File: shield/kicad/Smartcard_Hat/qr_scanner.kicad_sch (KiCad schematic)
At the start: 7 parts, among them J10 SFV12R-2STE1HLF

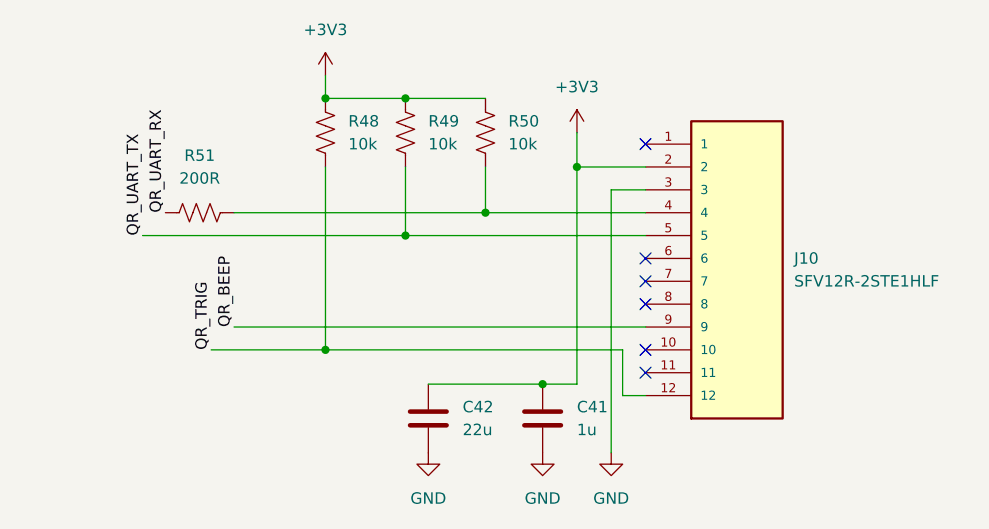
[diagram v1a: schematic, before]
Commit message: wip
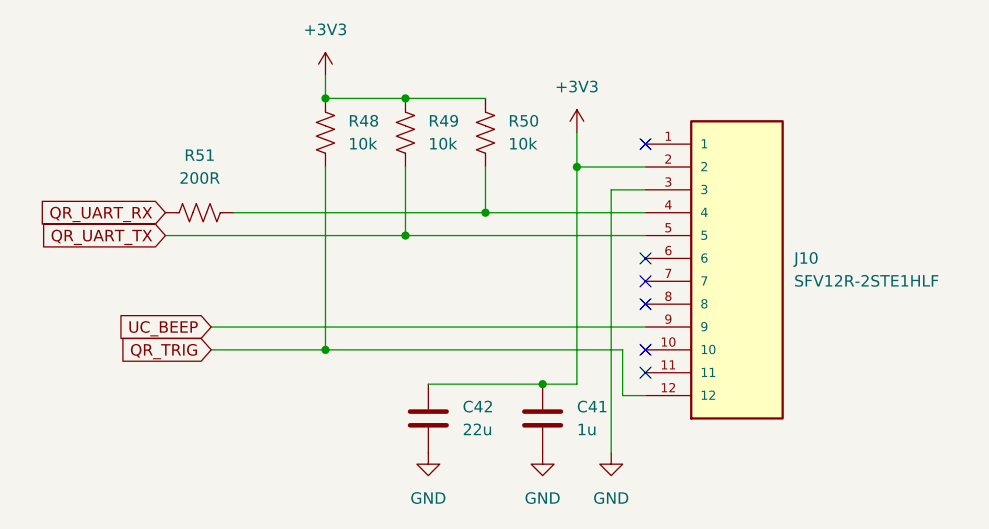
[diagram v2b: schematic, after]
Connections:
- net QR_BEEP renamed UC_BEEP
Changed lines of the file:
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@@
+	(wire
+		(pts
+			(xy 124.46 101.6) (xy 172.72 101.6)
+		)
+		(stroke
+			(width 0)
+			(type default)
+		)
+	)
 	(wire
 		(pts
@@
 	(wire
 		(pts
-			(xy 127 101.6) (xy 172.72 101.6)
-		)
-		(stroke
-			(width 0)
-			(type default)
-		)
-	)
-	(wire
-		(pts
 			(xy 127 88.9) (xy 154.94 88.9)
 		)
@@
 	(wire
 		(pts
-			(xy 116.84 91.44) (xy 146.05 91.44)
+			(xy 119.38 91.44) (xy 146.05 91.44)
 		)
 		(stroke
@@
 		)
 	)
-	(label "QR_UART_RX"
-		(at 119.38 88.9 90)
-		(fields_autoplaced yes)
-		(effects
-			(font
-				(size 1.27 1.27)
-			)
-			(justify left bottom)
-		)
-	)
-	(label "QR_TRIG"
-		(at 124.46 104.14 90)
-		(fields_autoplaced yes)
-		(effects
-			(font
-				(size 1.27 1.27)
-			)
-			(justify left bottom)
-		)
-	)
-	(label "QR_BEEP"
-		(at 127 101.6 90)
-		(fields_autoplaced yes)
-		(effects
-			(font
-				(size 1.27 1.27)
-			)
-			(justify left bottom)
-		)
-	)
-	(label "QR_UART_TX"
-		(at 116.84 91.44 90)
-		(fields_autoplaced yes)
-		(effects
-			(font
-				(size 1.27 1.27)
-			)
-			(justify left bottom)
-		)
-	)
+	(global_label "UC_BEEP"
+		(shape input)
+		(at 124.46 101.6 180)
+		(fields_autoplaced yes)
+		(effects
+			(font
+				(size 1.27 1.27)
+			)
+			(justify right)
+		)
+		(property "Intersheetrefs" "${INTERSHEET_REFS}"
+			(at 112.9736 101.6 0)
+			(effects
+				(font
+					(size 1.27 1.27)
+				)
+				(justify right)
+				(hide yes)
+			)
+		)
+	)
+	(global_label "QR_TRIG"
+		(shape input)
+		(at 124.46 104.14 180)
+		(fields_autoplaced yes)
+		(effects
+			(font
+				(size 1.27 1.27)
+			)
+			(justify right)
+		)
+		(property "Intersheetrefs" "${INTERSHEET_REFS}"
+			(at 113.6992 104.14 0)
+			(effects
+				(font
+					(size 1.27 1.27)
+				)
+				(justify right)
+				(hide yes)
+			)
+		)
+	)
+	(global_label "QR_UART_TX"
+		(shape input)
+		(at 119.38 91.44 180)
+		(fields_autoplaced yes)
+		(effects
+			(font
+				(size 1.27 1.27)
+			)
+			(justify right)
+		)
+		(property "Intersheetrefs" "${INTERSHEET_REFS}"
+			(at 104.9302 91.44 0)
+			(effects
+				(font
+					(size 1.27 1.27)
+				)
+				(justify right)
+				(hide yes)
+			)
+		)
+	)
+	(global_label "QR_UART_RX"
+		(shape input)
+		(at 119.38 88.9 180)
+		(fields_autoplaced yes)
+		(effects
+			(font
+				(size 1.27 1.27)
+			)
+			(justify right)
+		)
+		(property "Intersheetrefs" "${INTERSHEET_REFS}"
+			(at 104.6278 88.9 0)
+			(effects
+				(font
+					(size 1.27 1.27)
+				)
+				(justify right)
+				(hide yes)
+			)
+		)
+	)

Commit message: wip
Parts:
- R48, R49, R50, R51: footprint Resistor_SMD:R_0402_1005Metric_Pad0.72x0.64mm_HandSolder -> Resistor_SMD:R_0805_2012Metric_Pad1.20x1.40mm_HandSolder
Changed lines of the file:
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@@
 			)
 		)
-		(property "Footprint" "Resistor_SMD:R_0402_1005Metric_Pad0.72x0.64mm_HandSolder"
+		(property "Footprint" "Resistor_SMD:R_0805_2012Metric_Pad1.20x1.40mm_HandSolder"
 			(at 138.176 80.264 90)
 			(effects
@@
 			)
 		)
-		(property "Footprint" "Resistor_SMD:R_0402_1005Metric_Pad0.72x0.64mm_HandSolder"
+		(property "Footprint" "Resistor_SMD:R_0805_2012Metric_Pad1.20x1.40mm_HandSolder"
 			(at 123.444 87.884 90)
 			(effects
@@
 			)
 		)
-		(property "Footprint" "Resistor_SMD:R_0402_1005Metric_Pad0.72x0.64mm_HandSolder"
+		(property "Footprint" "Resistor_SMD:R_0805_2012Metric_Pad1.20x1.40mm_HandSolder"
 			(at 155.956 80.264 90)
 			(effects
@@
 			)
 		)
-		(property "Footprint" "Resistor_SMD:R_0402_1005Metric_Pad0.72x0.64mm_HandSolder"
+		(property "Footprint" "Resistor_SMD:R_0805_2012Metric_Pad1.20x1.40mm_HandSolder"
 			(at 147.066 80.264 90)
 			(effects
